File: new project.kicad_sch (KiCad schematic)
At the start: 4 parts

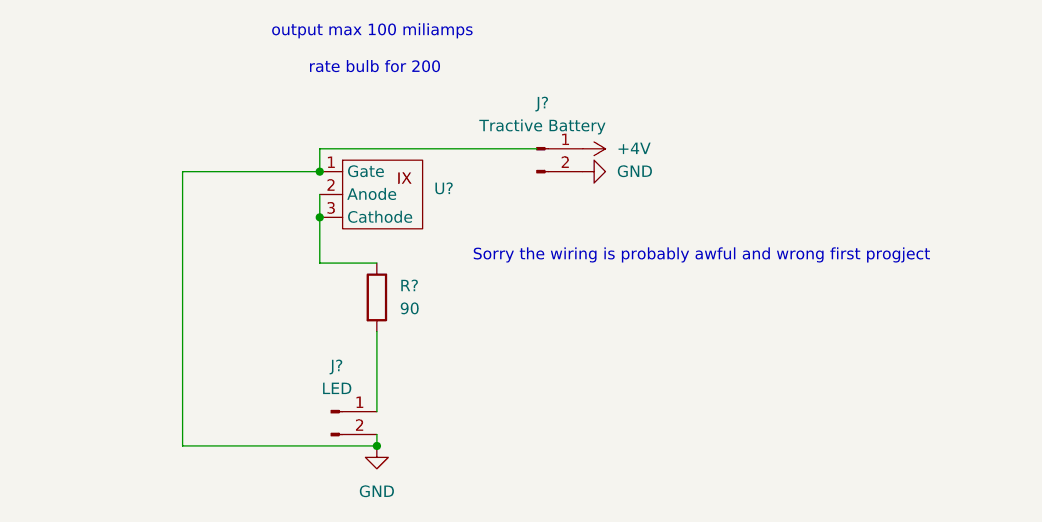
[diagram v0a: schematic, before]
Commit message: fixed
fix
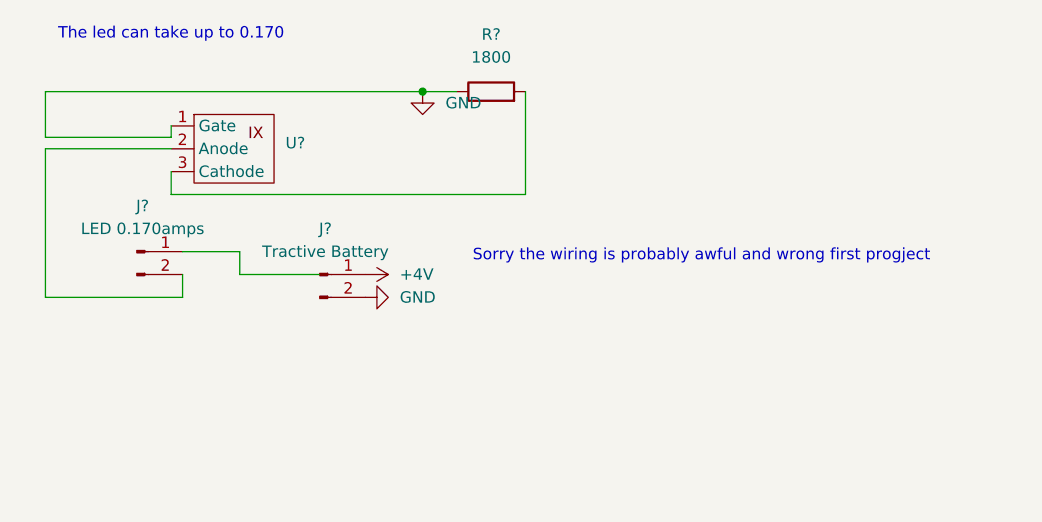
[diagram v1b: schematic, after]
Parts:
- removed J?: LED, symbol Connector:Conn_01x02_Pin
- removed R?: 90, symbol Device:R
- removed U?: ~, symbol IXCP10M90S:IXCP10M90S
- added J?: LED 0.170amps, symbol Connector:Conn_01x02_Pin
- added R?: 1800, symbol Device:R
- added U?: ~, symbol IXCP10M90S:IXCP10M90S
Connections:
- net GND: now also R?.1, U?.1 (Gate)
- new net: J?.2 (Pin_2), U?.2 (Anode)
- new net: R?.2, U?.3 (Cathode)
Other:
- note added: "The led can take up to 0.170"
- note removed: "output max 100 miliamps rate bulb for 200"
- moved on the sheet: J?

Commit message: footprints added
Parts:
- J? (x2), R?: footprint (none) -> Resistor_SMD:R_0201_0603Metric
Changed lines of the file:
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@@
 			)
 		)
-		(property "Footprint" ""
+		(property "Footprint" "Resistor_SMD:R_0201_0603Metric"
 			(at 55.88 113.03 0)
 			(effects
@@
 			)
 		)
-		(property "Footprint" ""
+		(property "Footprint" "Resistor_SMD:R_0201_0603Metric"
 			(at 35.56 110.49 0)
 			(effects
@@
 			)
 		)
-		(property "Footprint" ""
+		(property "Footprint" "Resistor_SMD:R_0201_0603Metric"
 			(at 74.93 94.488 90)
 			(effects

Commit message: all footprints added and they ready for wriing
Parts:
- U?: footprint (none) -> IXCP10M90S:IXCP10M90S
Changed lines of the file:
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@@
 			)
 		)
-		(property "Footprint" ""
+		(property "Footprint" "IXCP10M90S:IXCP10M90S"
 			(at 39.37 100.33 0)
 			(effects

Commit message: lkj
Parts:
- U?: footprint IXCP10M90S:IXCP10M90S -> Package_TO_SOT_SMD:TO-252-2
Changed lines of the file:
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@@
 			)
 		)
-		(property "Footprint" "IXCP10M90S:IXCP10M90S"
+		(property "Footprint" "Package_TO_SOT_SMD:TO-252-2"
 			(at 39.37 100.33 0)
 			(effects
